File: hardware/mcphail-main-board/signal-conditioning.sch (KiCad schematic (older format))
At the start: 66 parts, among them J1 INSECT DETECTION, J2 EMITTERS, J3 BREAKOUT, U1 MCP6004, U2 MCP6004, U3 TLV274, U4 MCP6001

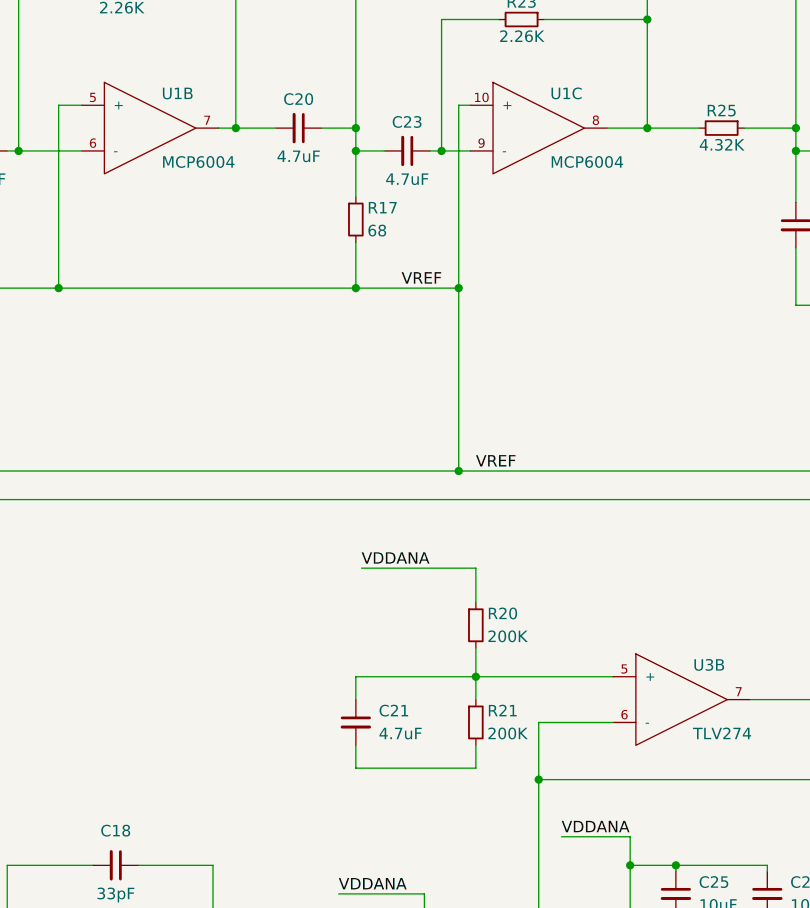
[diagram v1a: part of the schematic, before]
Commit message: Commit.
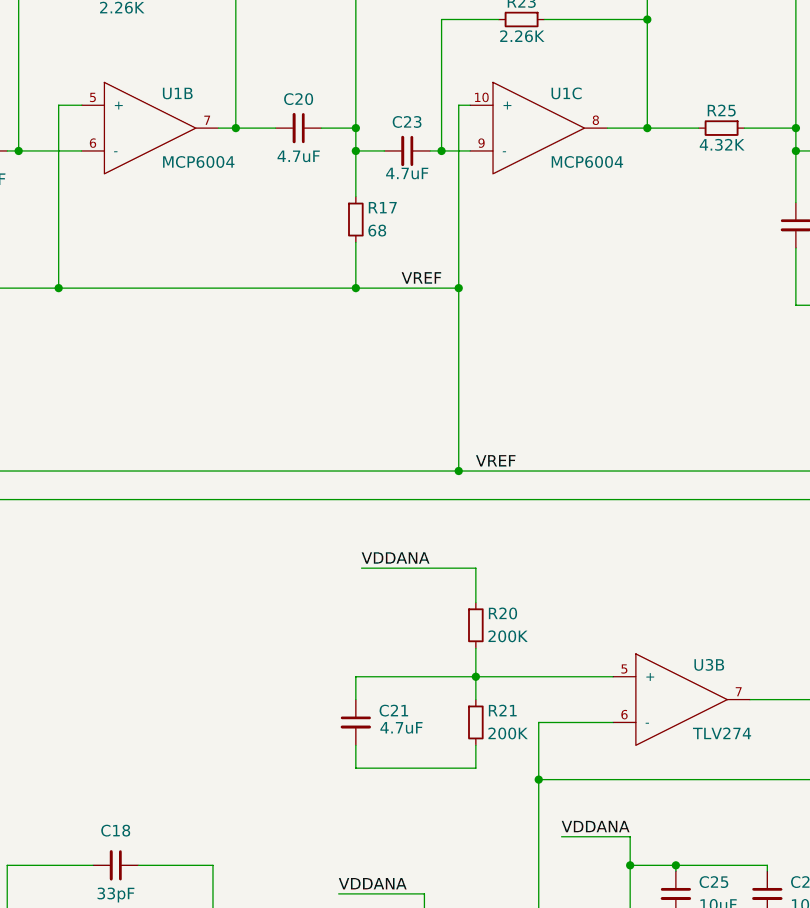
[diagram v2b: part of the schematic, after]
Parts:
- C20, C21, C23, C24: MF_Name Taiyo Yuden -> Samsung; MF_PN UMK316AB7475KL-T -> CL31B475KBHNNNE; S1_PN 587-2994-1-ND -> 1276-2789-1-ND
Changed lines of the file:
@@
 EESchema Schematic File Version 2
 LIBS:wickerlib
-LIBS:mcphail-main-board-cache
 EELAYER 25 0
 EELAYER END
@@
 $EndComp
 $Comp
-L CAP-CER-4.7UF-50V-X7R-1206 C20
-U 1 1 596FCAF3
-P 8775 3925
-F 0 "C20" V 8650 3925 50  0000 C CNN
-F 1 "4.7uF" V 8900 3925 50  0000 C CNN
-F 2 "Wickerlib:RLC-1206-SMD" H 9400 3525 50  0001 C CIN
-F 3 "http://ds.yuden.co.jp/TYCOMPAS/ut/detail.do?productNo=UMK316AB7475KL-T&fileName=UMK316AB7475KL-T_SS&mode=specSheetDownload" H 9125 3700 50  0001 C CNN
-F 4 "CAP CER 4.7UF 50V X7R 1206" H 9450 3600 50  0001 C CIN "Description"
-F 5 "Taiyo Yuden" H 8975 3425 50  0001 C CIN "MF_Name"
-F 6 "UMK316AB7475KL-T" H 9650 3425 50  0001 C CIN "MF_PN"
-F 7 "Digikey" H 8875 3325 50  0001 C CIN "S1_Name"
-F 8 "587-2994-1-ND" H 9575 3325 50  0001 C CIN "S1_PN"
-	1    8775 3925
-	0    1    1    0
-$EndComp
-$Comp
 L CAP-CER-4.7UF-50V-X7R-1206 C24
 U 1 1 596FCAFF
@@
 F 1 "4.7uF" V 9875 3100 50  0000 C CNN
 F 2 "Wickerlib:RLC-1206-SMD" H 10375 2700 50  0001 C CIN
-F 3 "http://ds.yuden.co.jp/TYCOMPAS/ut/detail.do?productNo=UMK316AB7475KL-T&fileName=UMK316AB7475KL-T_SS&mode=specSheetDownload" H 10100 2875 50  0001 C CNN
+F 3 "http://www.samsungsem.com/kr/support/product-search/mlcc/CL31B475KBHNNNE.jsp" H 10100 2875 50  0001 C CNN
 F 4 "CAP CER 4.7UF 50V X7R 1206" H 10425 2775 50  0001 C CIN "Description"
-F 5 "Taiyo Yuden" H 9950 2600 50  0001 C CIN "MF_Name"
-F 6 "UMK316AB7475KL-T" H 10625 2600 50  0001 C CIN "MF_PN"
+F 5 "Samsung" H 9950 2600 50  0001 C CIN "MF_Name"
+F 6 "CL31B475KBHNNNE" H 10625 2600 50  0001 C CIN "MF_PN"
 F 7 "Digikey" H 9850 2500 50  0001 C CIN "S1_Name"
-F 8 "587-2994-1-ND" H 10550 2500 50  0001 C CIN "S1_PN"
+F 8 "1276-2789-1-ND" H 10550 2500 50  0001 C CIN "S1_PN"
 	1    9750 3100
 	0    1    1    0
@@
 P 9250 4025
 F 0 "C23" V 9125 4025 50  0000 C CNN
-F 1 "4.7uF" V 9375 4025 50  0000 C CNN
-F 2 "Wickerlib:RLC-1206-SMD" H 9875 3625 50  0001 C CIN
-F 3 "http://ds.yuden.co.jp/TYCOMPAS/ut/detail.do?productNo=UMK316AB7475KL-T&fileName=UMK316AB7475KL-T_SS&mode=specSheetDownload" H 9600 3800 50  0001 C CNN
-F 4 "CAP CER 4.7UF 50V X7R 1206" H 9925 3700 50  0001 C CIN "Description"
-F 5 "Taiyo Yuden" H 9450 3525 50  0001 C CIN "MF_Name"
-F 6 "UMK316AB7475KL-T" H 10125 3525 50  0001 C CIN "MF_PN"
-F 7 "Digikey" H 9350 3425 50  0001 C CIN "S1_Name"
-F 8 "587-2994-1-ND" H 10050 3425 50  0001 C CIN "S1_PN"
+F 1 "4.7uF" V 9350 4025 50  0000 C CNN
+F 2 "Wickerlib:RLC-1206-SMD" H 10375 2700 50  0001 C CIN
+F 3 "http://www.samsungsem.com/kr/support/product-search/mlcc/CL31B475KBHNNNE.jsp" H 10100 2875 50  0001 C CNN
+F 4 "CAP CER 4.7UF 50V X7R 1206" H 10425 2775 50  0001 C CIN "Description"
+F 5 "Samsung" H 9950 2600 50  0001 C CIN "MF_Name"
+F 6 "CL31B475KBHNNNE" H 10625 2600 50  0001 C CIN "MF_PN"
+F 7 "Digikey" H 9850 2500 50  0001 C CIN "S1_Name"
+F 8 "1276-2789-1-ND" H 10550 2500 50  0001 C CIN "S1_PN"
 	1    9250 4025
 	0    1    1    0
@@
 P 9025 6525
 F 0 "C21" H 9125 6575 50  0000 L CNN
-F 1 "4.7uF" H 9125 6475 50  0000 L CNN
-F 2 "Wickerlib:RLC-1206-SMD" H 9650 6125 50  0001 C CIN
-F 3 "http://ds.yuden.co.jp/TYCOMPAS/ut/detail.do?productNo=UMK316AB7475KL-T&fileName=UMK316AB7475KL-T_SS&mode=specSheetDownload" H 9375 6300 50  0001 C CNN
-F 4 "CAP CER 4.7UF 50V X7R 1206" H 9700 6200 50  0001 C CIN "Description"
-F 5 "Taiyo Yuden" H 9225 6025 50  0001 C CIN "MF_Name"
-F 6 "UMK316AB7475KL-T" H 9900 6025 50  0001 C CIN "MF_PN"
-F 7 "Digikey" H 9125 5925 50  0001 C CIN "S1_Name"
-F 8 "587-2994-1-ND" H 9825 5925 50  0001 C CIN "S1_PN"
+F 1 "4.7uF" H 9225 6500 50  0000 C CNN
+F 2 "Wickerlib:RLC-1206-SMD" H 10375 2700 50  0001 C CIN
+F 3 "http://www.samsungsem.com/kr/support/product-search/mlcc/CL31B475KBHNNNE.jsp" H 10100 2875 50  0001 C CNN
+F 4 "CAP CER 4.7UF 50V X7R 1206" H 10425 2775 50  0001 C CIN "Description"
+F 5 "Samsung" H 9950 2600 50  0001 C CIN "MF_Name"
+F 6 "CL31B475KBHNNNE" H 10625 2600 50  0001 C CIN "MF_PN"
+F 7 "Digikey" H 9850 2500 50  0001 C CIN "S1_Name"
+F 8 "1276-2789-1-ND" H 10550 2500 50  0001 C CIN "S1_PN"
 	1    9025 6525
 	1    0    0    -1
@@
 Text Label 12425 8325 0    50   ~ 0
 VDDANA
+$Comp
+L CAP-CER-4.7UF-50V-X7R-1206 C20
+U 1 1 596FCAF3
+P 8775 3925
+F 0 "C20" V 8650 3925 50  0000 C CNN
+F 1 "4.7uF" V 8900 3925 50  0000 C CNN
+F 2 "Wickerlib:RLC-1206-SMD" H 10375 2700 50  0001 C CIN
+F 3 "http://www.samsungsem.com/kr/support/product-search/mlcc/CL31B475KBHNNNE.jsp" H 10100 2875 50  0001 C CNN
+F 4 "CAP CER 4.7UF 50V X7R 1206" H 10425 2775 50  0001 C CIN "Description"
+F 5 "Samsung" H 9950 2600 50  0001 C CIN "MF_Name"
+F 6 "CL31B475KBHNNNE" H 10625 2600 50  0001 C CIN "MF_PN"
+F 7 "Digikey" H 9850 2500 50  0001 C CIN "S1_Name"
+F 8 "1276-2789-1-ND" H 10550 2500 50  0001 C CIN "S1_PN"
+	1    8775 3925
+	0    1    1    0
+$EndComp
 $EndSCHEMATC
